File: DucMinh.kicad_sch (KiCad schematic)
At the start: 51 parts, among them J5 USB_B_Micro, J8 Conn_01x04, SW1 SW_Push, U1 STM32F103C8T6, U2 AMS1117-3.3, U3 LM2596SX-5.0/NOPB, U4 TMC2209_SILENTSTEPSTICK, Y1 8 MHz, Y3 32.768 kHz

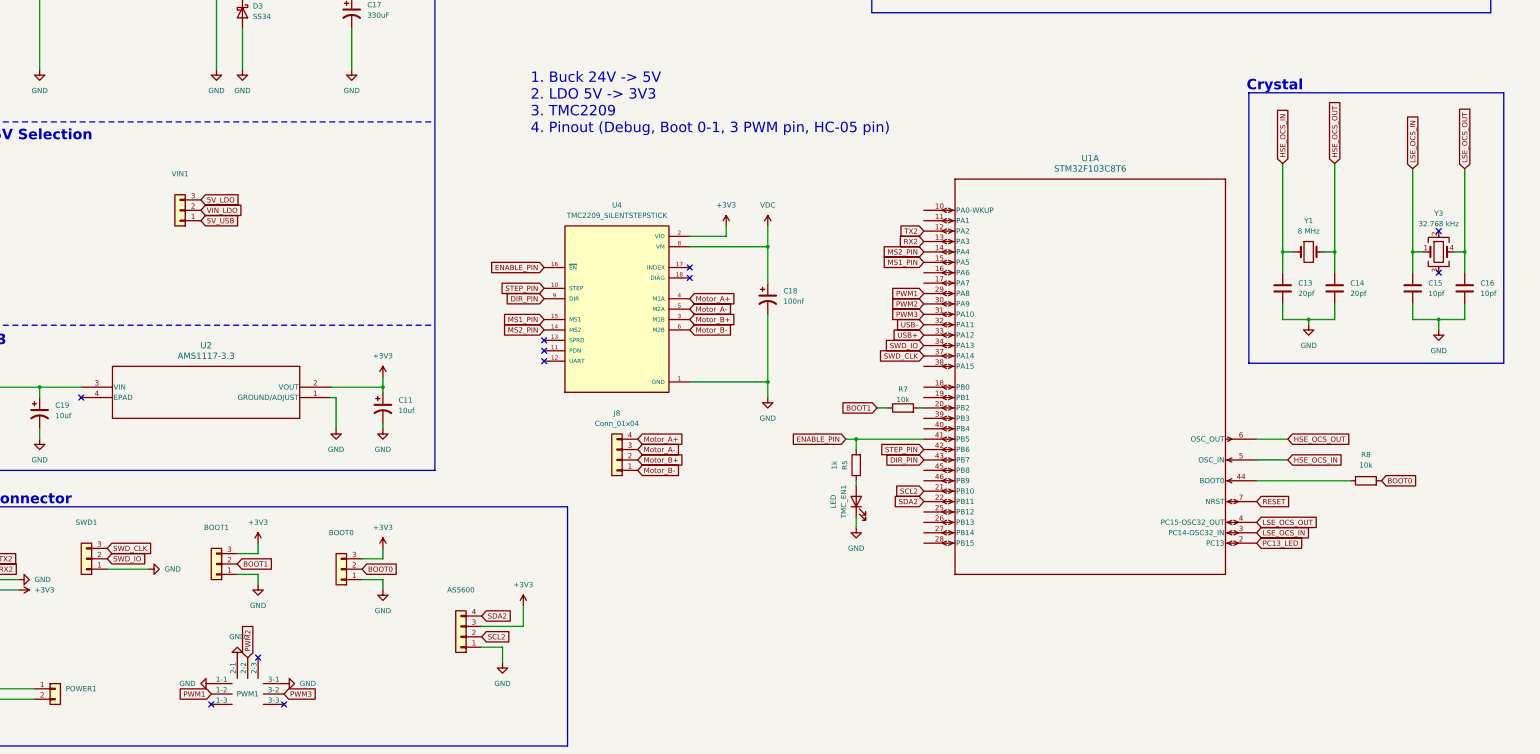
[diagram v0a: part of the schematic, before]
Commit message: .
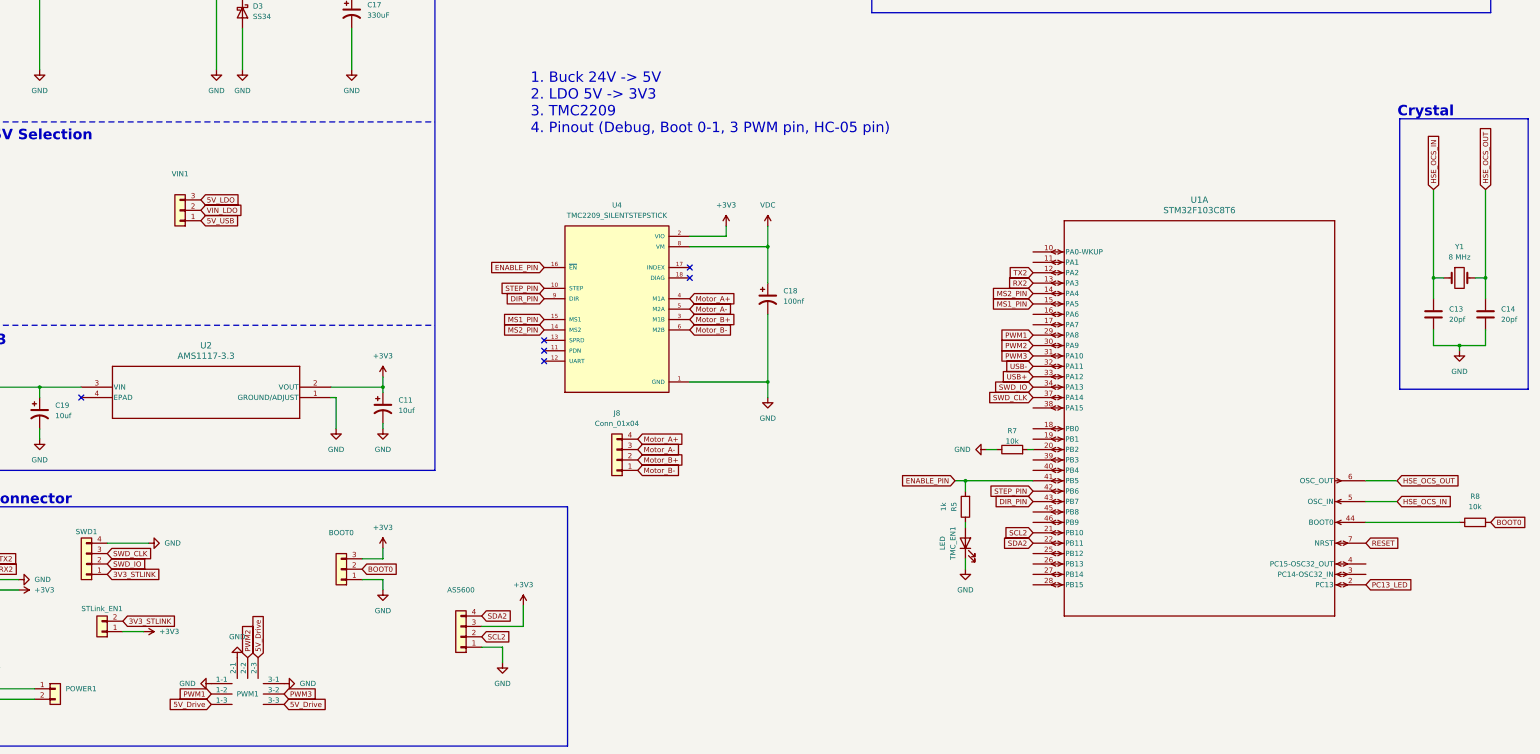
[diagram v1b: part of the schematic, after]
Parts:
- removed BOOT1: BOOT1, ul_switch-SS12D00:tue_SS12D00_3P_2.5mm, symbol Connector_Generic:Conn_01x03
- removed C15, C16: 10pf, Capacitor_SMD:C_0603_1608Metric_Pad1.08x0.95mm_HandSolder, symbol Device:C
- removed SWD1: SWD, Connector_PinHeader_2.54mm:PinHeader_1x03_P2.54mm_Vertical, symbol Connector_Generic:Conn_01x03
- removed Y3: 32.768 kHz, ul_crytsal_mc306:SOJ_MC-306_EPS, symbol Device:Crystal_GND23
- added STLink_EN1: POWER, Connector_PinHeader_2.54mm:PinHeader_1x02_P2.54mm_Vertical, symbol Connector_Generic:Conn_01x02
- added SWD1: Conn_01x04, Connector_JST:JST_XH_B4B-XH-A_1x04_P2.50mm_Vertical, symbol Connector_Generic:Conn_01x04
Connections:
- net BOOT1 is gone; now on net GND: R7.1
- net +3V3: now also STLink_EN1.1 (Pin_1)
- net GND: now also SWD1.4 (Pin_4)
- net SWD_CLK: now also SWD1.3 (Pin_3)
- net SWD_IO: now also SWD1.2 (Pin_2)
- net 5V_Drive: now reaches PWM1.1-3
- net 5V_Drive: now also PWM1.2-3, PWM1.3-3
- net LSE_OCS_IN: no longer names the net of U1.3 (PC14-OSC32_IN)
- net LSE_OCS_OUT: no longer names the net of U1.4 (PC15-OSC32_OUT)
- new net 3V3_STLINK: STLink_EN1.2 (Pin_2), SWD1.1 (Pin_1)
- no-connect marks 15 -> 10
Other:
- moved on the sheet: C13, C14, R5, R7, R8, TMC_EN1, U1A, Y1
